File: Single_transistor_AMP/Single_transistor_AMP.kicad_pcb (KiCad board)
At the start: 2 copper layers, 40 x 46 mm, 9 parts, among them P1 Signal_IN, P2 Signal_OUT, Q1 BC547

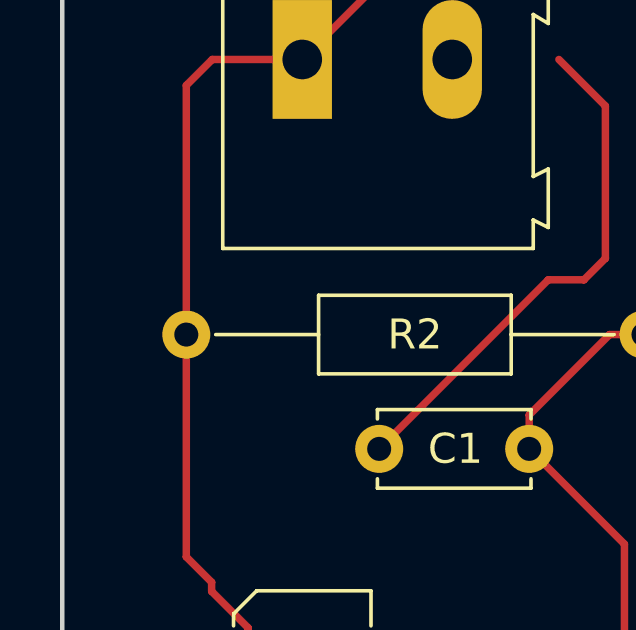
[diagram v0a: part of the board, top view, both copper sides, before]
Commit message: Kursa_darbs_PCB
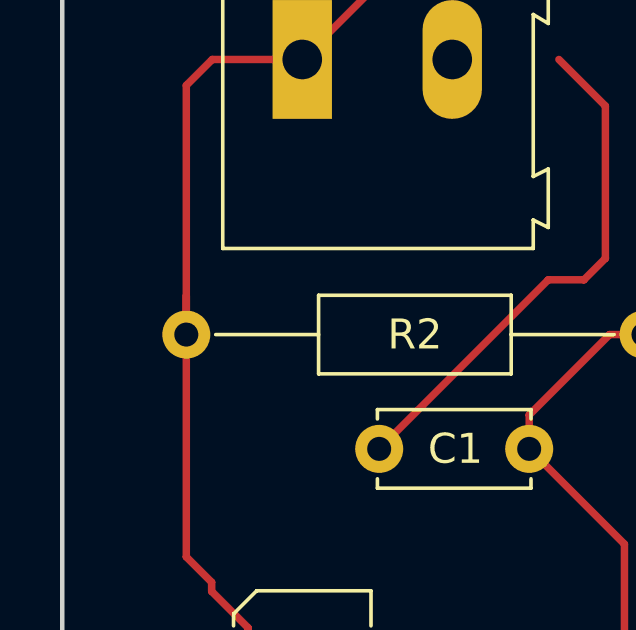
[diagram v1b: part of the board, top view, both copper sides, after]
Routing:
- net GND: track 58.2 -> 59.5 mm
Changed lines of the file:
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@@
     (thickness 1.6)
     (drawings 4)
-    (tracks 44)
+    (tracks 45)
     (zones 0)
     (modules 9)
@@
       (outputformat 1)
       (mirror false)
-      (drillshape 1)
+      (drillshape 0)
       (scaleselection 1)
-      (outputdirectory ""))
+      (outputdirectory "C:/Users/Alfs Briksis/Desktop/testproject/PCB-kurss/Single_transistor_AMP/"))
   )
   (net 0 "")
@@
   (segment (start 78.105 87.63) (end 78.105 82.55) (width 0.25) (layer F.Cu) (net 3))
   (segment (start 78.105 82.55) (end 76.555 81) (width 0.25) (layer F.Cu) (net 3))
+  (segment (start 64.135 90.17) (end 64.135 88.865) (width 0.25) (layer F.Cu) (net 4))
   (segment (start 71 78) (end 68 81) (width 0.25) (layer F.Cu) (net 4))
   (segment (start 80.88863 78) (end 71 78) (width 0.25) (layer F.Cu) (net 4))
